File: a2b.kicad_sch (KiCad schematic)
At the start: 10 parts, among them J1 RAPC722X, J2 PPPC031LFBN-RC, J3 NMJ6HCD2, J4 PPPC031LFBN-RC, J5 NMJ6HCD2, J6 PPPC031LFBN-RC, SW1 ANT21SECQE, SW2 ANT21SECQE

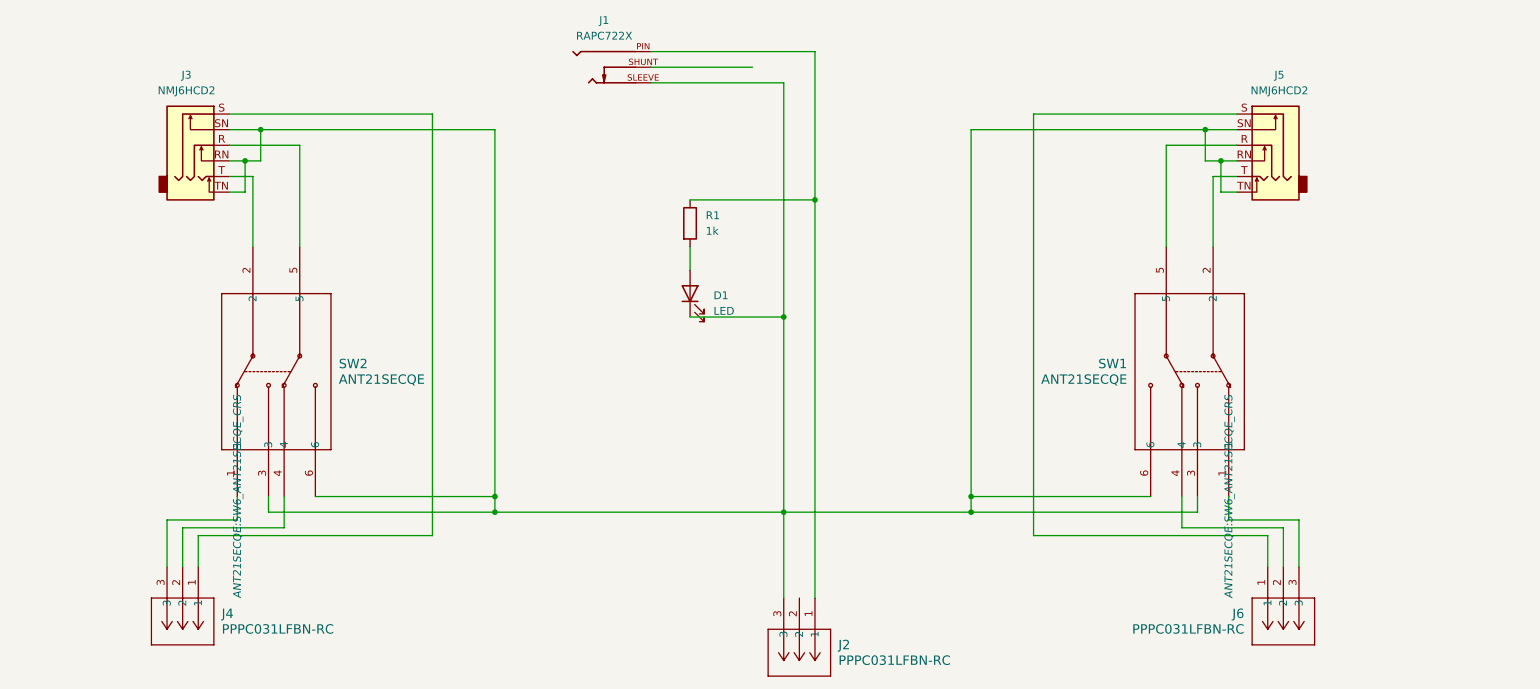
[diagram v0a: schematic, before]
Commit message: UPDATE PCB
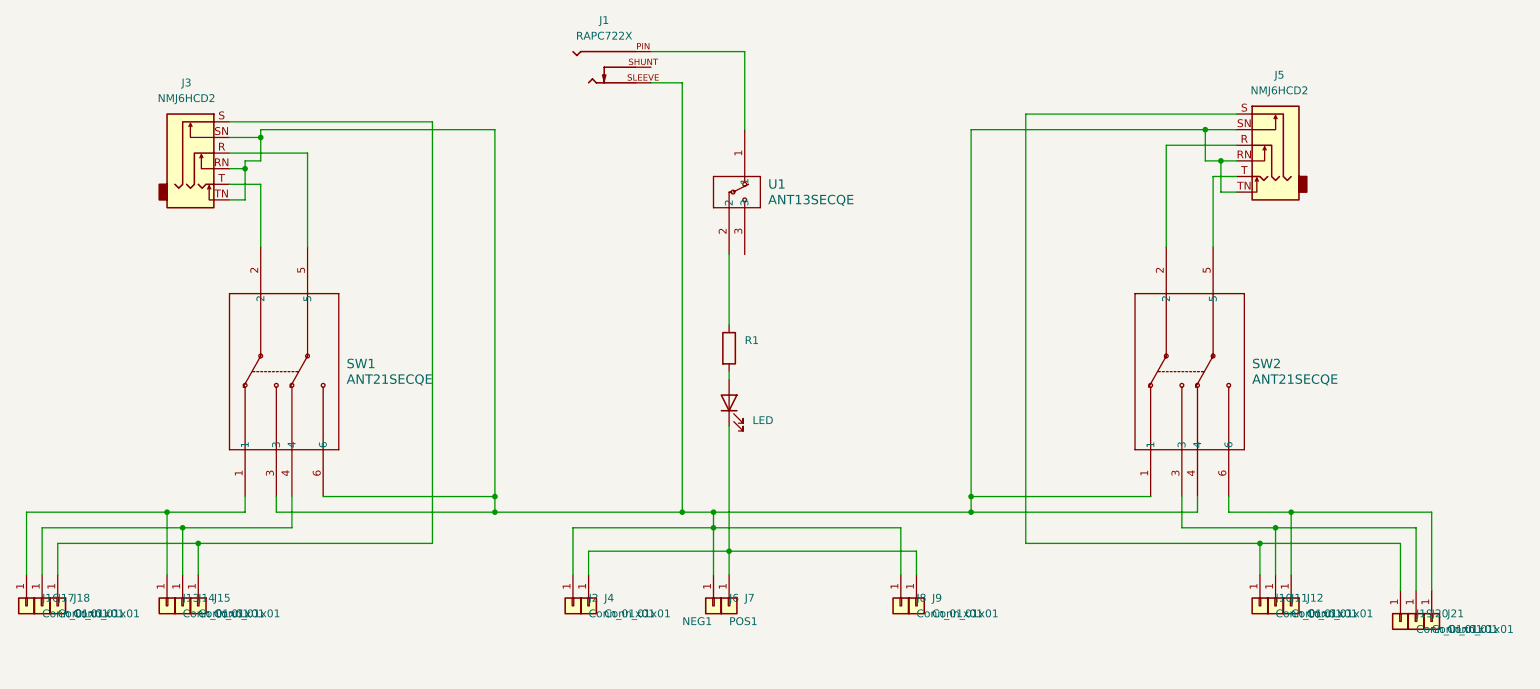
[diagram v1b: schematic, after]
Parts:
- removed J2, J4, J6: PPPC031LFBN-RC, PPPC031LFBN:CONN_PPPC031LFBN-RC_SUL, symbol PPPC031LFBN_RC:PPPC031LFBN-RC
- removed SW1, SW2: ANT21SECQE, ANT21SECQE:SW6_ANT21SECQE_CRS, symbol 2026-04-30_17-37-32:ANT21SECQE
- added J10, J11, J12, J13, J14, J15, J16, J17, J18, J19, J20, J21, J8, J9: Conn_01x01, TestPoint:TestPoint_THTPad_D2.0mm_Drill1.0mm, symbol Connector_Generic:Conn_01x01
- added J2, J4: Conn_01x01, TestPoint:TestPoint_Pad_D1.5mm, symbol Connector_Generic:Conn_01x01
- added J6: NEG1, TestPoint:TestPoint_THTPad_D2.0mm_Drill1.0mm, symbol Connector_Generic:Conn_01x01
- added J7: POS1, TestPoint:TestPoint_THTPad_D2.0mm_Drill1.0mm, symbol Connector_Generic:Conn_01x01
- added SW1, SW2: ANT21SECQE, ANT21SECQE:SW6_ANT21SECQE_CRS, symbol ANT21SECQE:ANT21SECQE
- added U1: ANT13SECQE, footprints:ANT13SEC_CRS, symbol ANT13SECQE:ANT13SECQE
- R1: footprint Resistor_THT:R_Bare_Metal_Element_L12.4mm_W4.8mm_P11.40mm -> Resistor_THT:R_Axial_DIN0207_L6.3mm_D2.5mm_P10.16mm_Horizontal
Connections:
- net at R1.1: now also U1.2; no longer J1.PIN
- net at J5.T: now also SW2.5
- net at J1.SLEEVE, J3.RN, J3.SN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: now also J2.1 (Pin_1), J6.1 (Pin_1), J8.1 (Pin_1), SW1.3, SW1.6, SW2.1, SW2.4; no longer D1.1 (K)
- net at J5.R: now also SW2.2
- net at J5.S: now also J10.1 (Pin_1), J19.1 (Pin_1)
- net at J3.R: now also SW1.5
- net at J3.S: now also J15.1 (Pin_1), J18.1 (Pin_1)
- net at J3.T: now also SW1.2
- new net: J11.1 (Pin_1), J20.1 (Pin_1), SW2.3
- new net: D1.1 (K), J4.1 (Pin_1), J7.1 (Pin_1), J9.1 (Pin_1)
- new net: J1.PIN, U1.1
- new net: J12.1 (Pin_1), J21.1 (Pin_1), SW2.6
- new net: J14.1 (Pin_1), J17.1 (Pin_1), SW1.4
- new net: J13.1 (Pin_1), J16.1 (Pin_1), SW1.1
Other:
- moved on the sheet: J3
